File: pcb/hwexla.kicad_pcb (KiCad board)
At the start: 4 copper layers, 53.5 x 53 mm, 82 parts, among them J1 DB25_Male, J2 Conn_01x03, J3 AVR-ISP-6, J4 Conn_01x06, J5 Conn_01x04, K1 HFD2/005, Q1 BT148, Q2 2N7002, Q3 2N7002, Q4 2N7002, Q5 2N7002, Q6 2N7002, Q7 BT148, Q8 BT148, SW1 SW_Push, U1 ATmega8A-AU, U2 RR112-1, U3 KA78M05_TO252

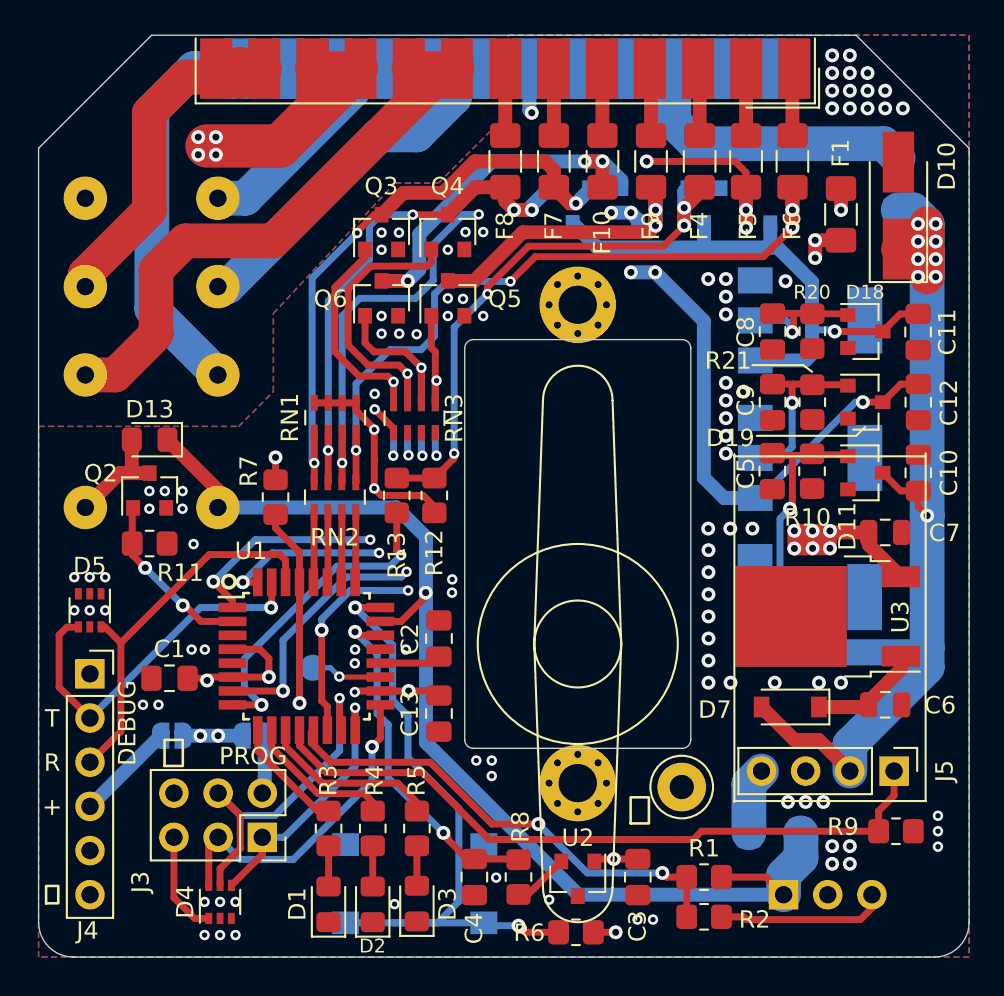
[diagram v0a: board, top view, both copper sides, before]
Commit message: Migrate to KiCad 6.
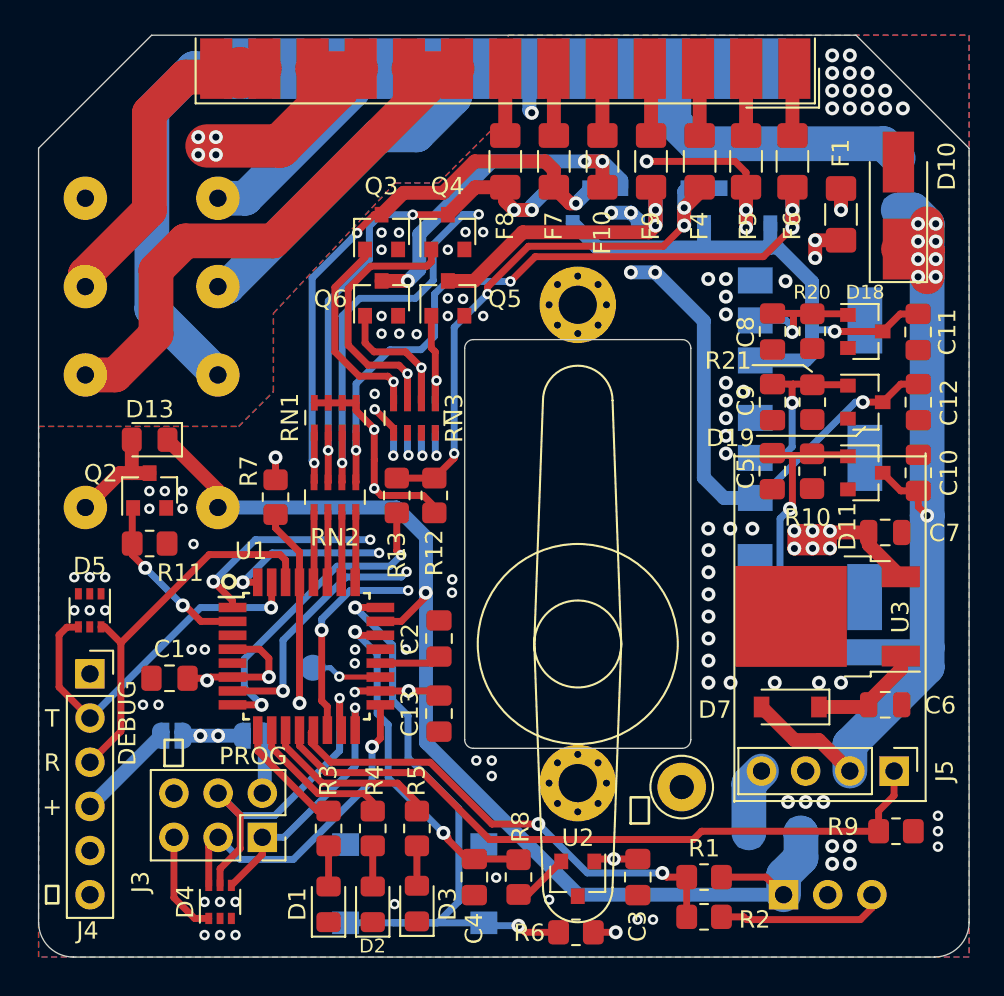
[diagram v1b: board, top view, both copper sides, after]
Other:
- net class Default removed
- net class Trakce removed
